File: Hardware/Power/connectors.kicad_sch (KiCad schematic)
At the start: 3 parts, among them J1 Conn_02x23_Odd_Even, J2 Screw_Terminal_01x03, J3 Conn_02x23_Odd_Even

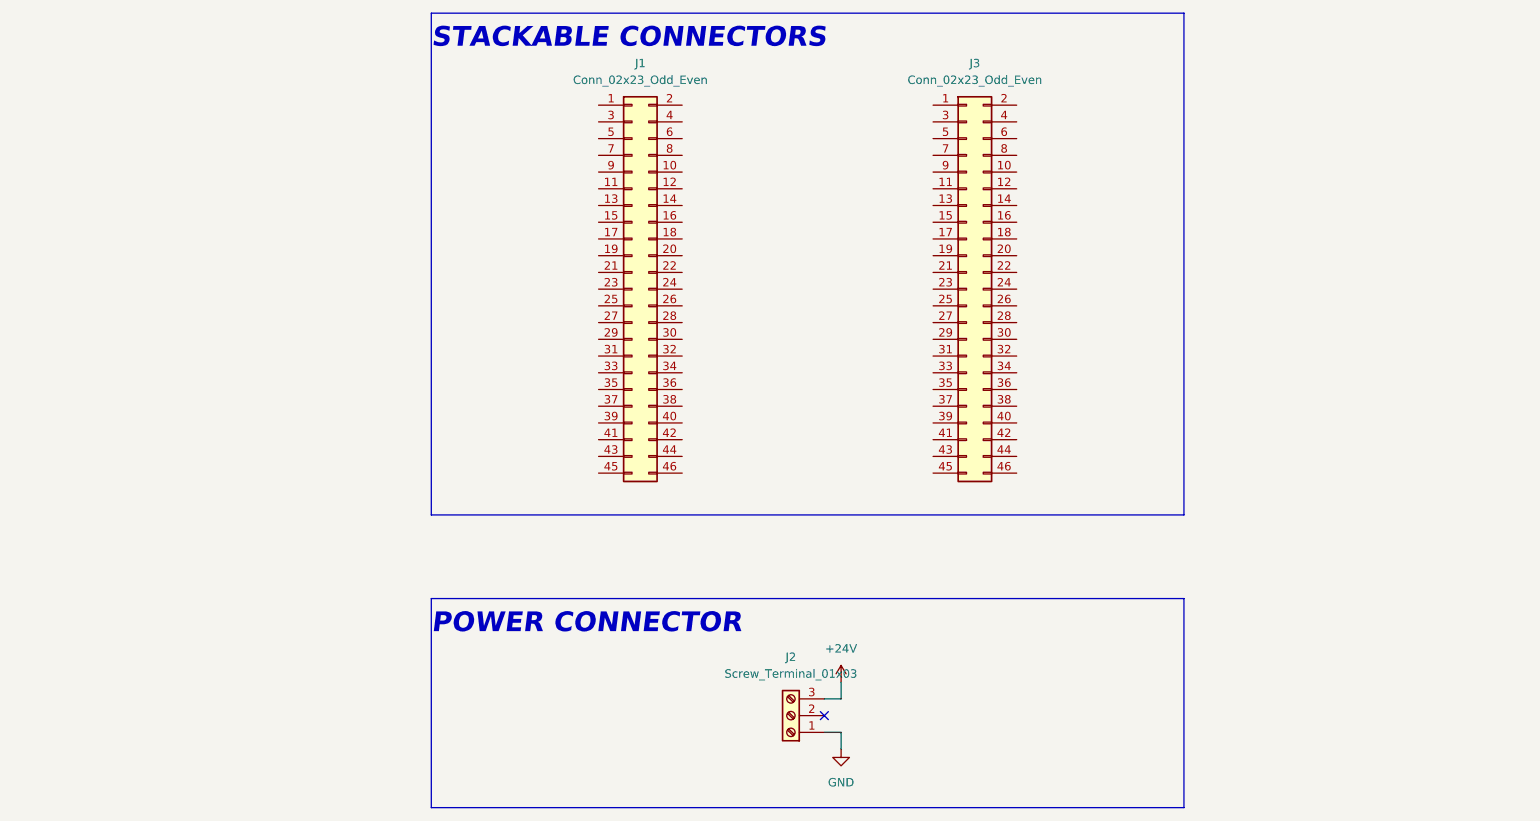
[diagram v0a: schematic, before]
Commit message: schematic update & pcb update
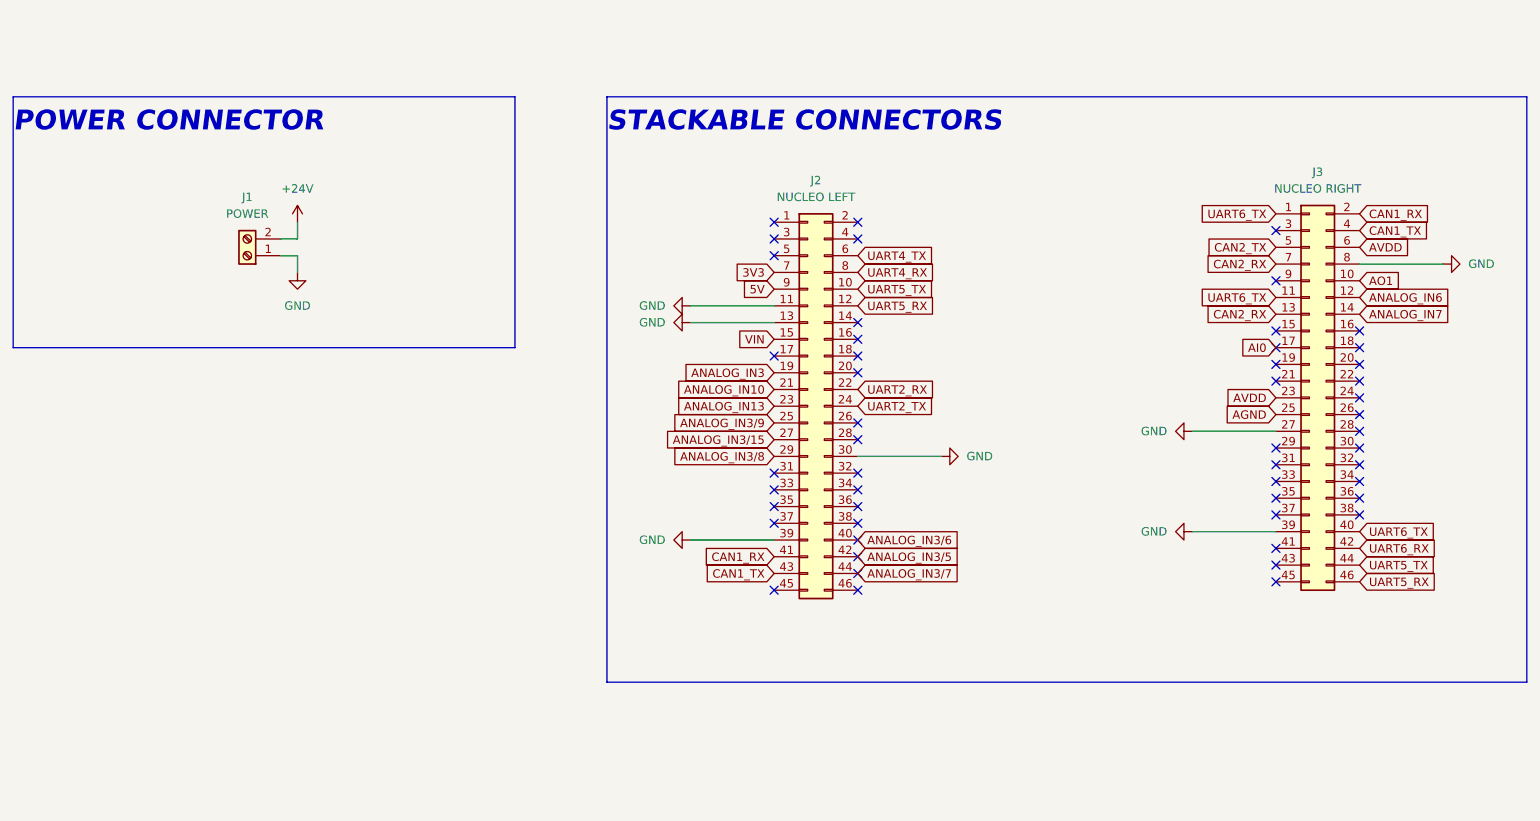
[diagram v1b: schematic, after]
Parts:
- removed J1: Conn_02x23_Odd_Even, PLC_STM_Power:PRT12790, symbol Connector_Generic:Conn_02x23_Odd_Even
- removed J2: Screw_Terminal_01x03, PLC_STM_Power:TBC05031GG, symbol Connector:Screw_Terminal_01x03
- added J1: POWER, PLC_STM:1725656, symbol Connector:Screw_Terminal_01x02
- added J2: NUCLEO LEFT, PLC_STM_Power:PRT12790, symbol Connector_Generic:Conn_02x23_Odd_Even
- J3: value Conn_02x23_Odd_Even -> NUCLEO RIGHT
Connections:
- net +24V: now also J1.2 (Pin_2)
- net GND: now also J3.27 (Pin_27), J3.39 (Pin_39), J3.8 (Pin_8), J1.1 (Pin_1), J2.11 (Pin_11), J2.13 (Pin_13), J2.30 (Pin_30), J2.39 (Pin_39)
- net UART6_TX: now reaches J3.1 (Pin_1)
- net UART6_TX: now also J3.11 (Pin_11), J3.40 (Pin_40)
- net AO1: now reaches J3.10 (Pin_10)
- net ANALOG_IN6: now reaches J3.12 (Pin_12)
- net CAN2_RX: now reaches J3.13 (Pin_13)
- net CAN2_RX: now also J3.7 (Pin_7)
- net ANALOG_IN7: now reaches J3.14 (Pin_14)
- net AI0: now reaches J3.17 (Pin_17)
- net CAN1_RX: now reaches J3.2 (Pin_2)
- net CAN1_RX: now also J2.41 (Pin_41)
- net AVDD: now reaches J3.23 (Pin_23)
- net AVDD: now also J3.6 (Pin_6)
- net AGND: now reaches J3.25 (Pin_25)
- net CAN1_TX: now reaches J3.4 (Pin_4)
- net CAN1_TX: now also J2.43 (Pin_43)
- net UART6_RX: now reaches J3.42 (Pin_42)
- net UART5_TX: now reaches J3.44 (Pin_44)
- net UART5_TX: now also J2.10 (Pin_10)
- net UART5_RX: now reaches J3.46 (Pin_46)
- net UART5_RX: now also J2.12 (Pin_12)
- net CAN2_TX: now reaches J3.5 (Pin_5)
- new net 3V3: J2.7 (Pin_7)
- new net 5V: J2.9 (Pin_9)
- new net ANALOG_IN10: J2.21 (Pin_21)
- new net ANALOG_IN13: J2.23 (Pin_23)
- new net ANALOG_IN3: J2.19 (Pin_19)
- new net ANALOG_IN3/15: J2.27 (Pin_27)
- new net ANALOG_IN3/5: J2.42 (Pin_42)
- new net ANALOG_IN3/6: J2.40 (Pin_40)
- new net ANALOG_IN3/7: J2.44 (Pin_44)
- new net ANALOG_IN3/8: J2.29 (Pin_29)
- new net ANALOG_IN3/9: J2.25 (Pin_25)
- new net UART2_RX: J2.22 (Pin_22)
- new net UART2_TX: J2.24 (Pin_24)
- new net UART4_RX: J2.8 (Pin_8)
- new net UART4_TX: J2.6 (Pin_6)
- new net VIN: J2.15 (Pin_15)
- no-connect marks 1 -> 51
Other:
- moved on the sheet: J3
